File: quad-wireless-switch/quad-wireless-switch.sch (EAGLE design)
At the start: 69 parts, among them IC1 LM2937IMP-3.3, Q1 DN2625K4-G, Q2 SI2323DS-T1-E3, Q3 IRL520, Q4 IRL520, Q5 IRL520, Q6 IRL520, U1 ATMEGA328P_TQFP

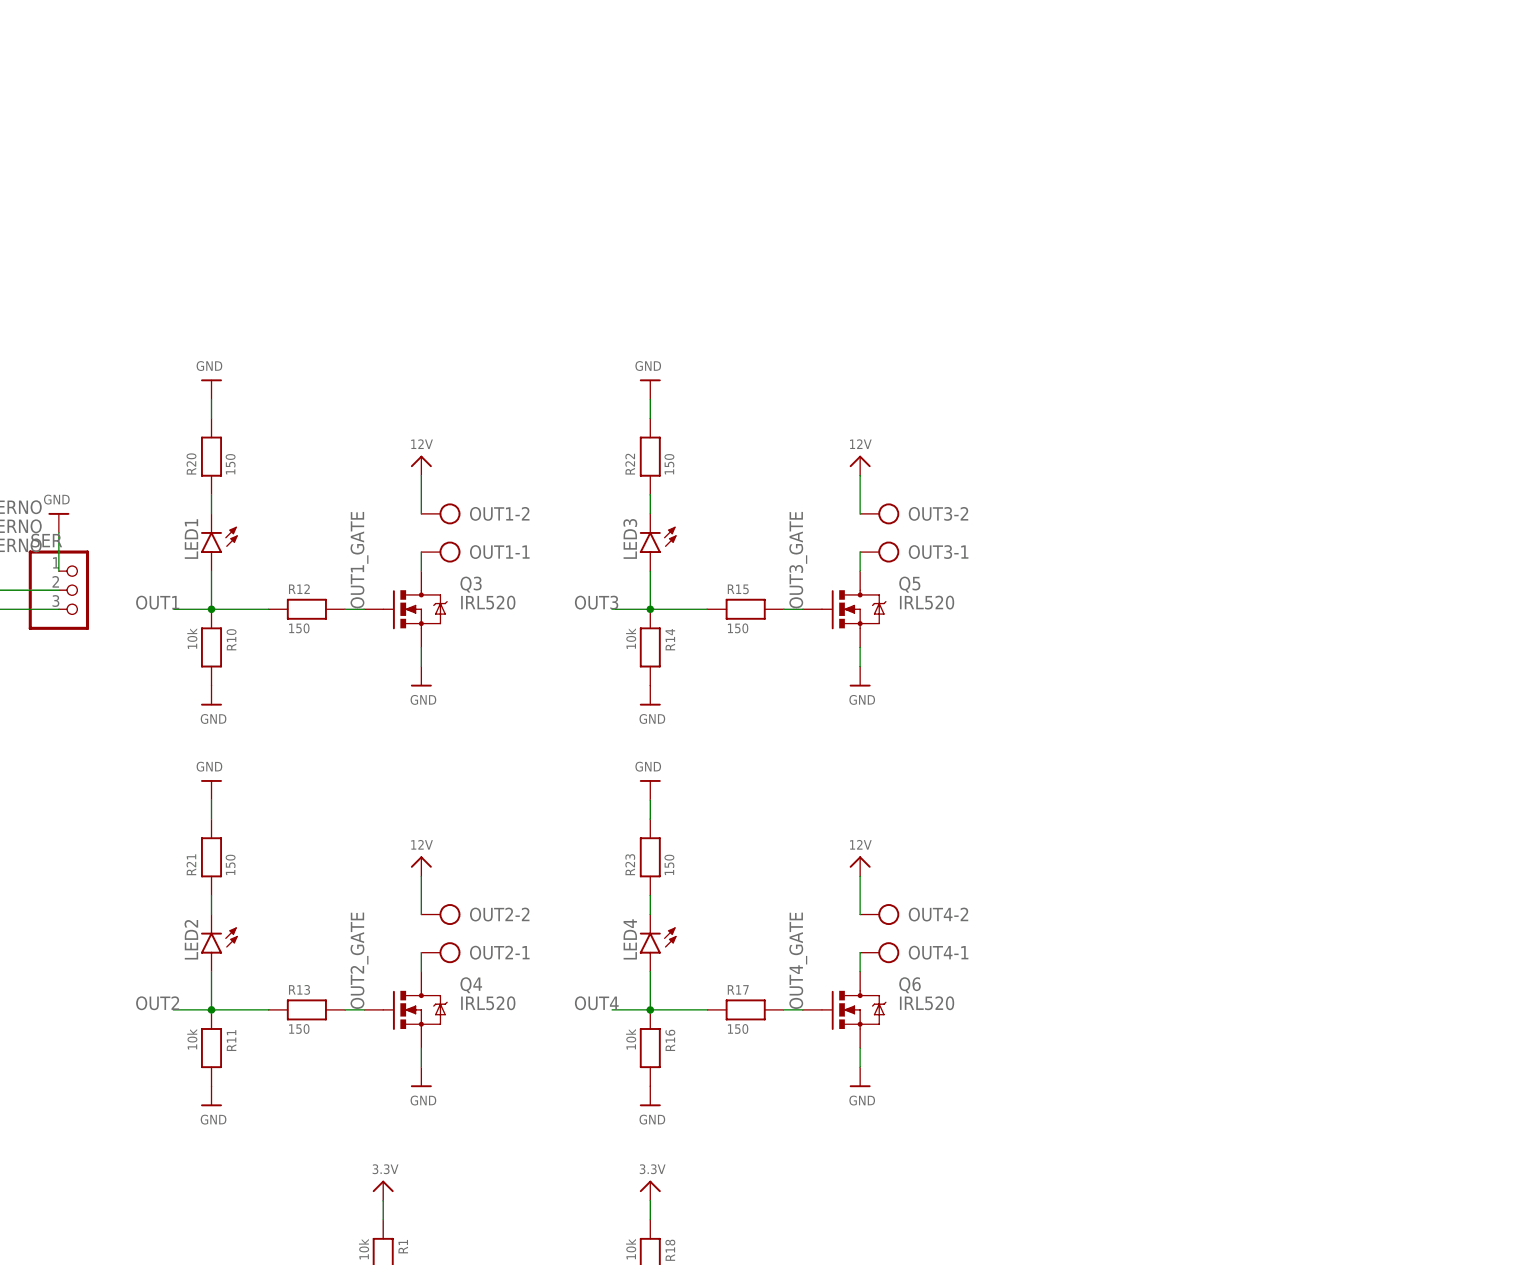
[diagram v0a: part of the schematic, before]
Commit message: quad wireless switch wip
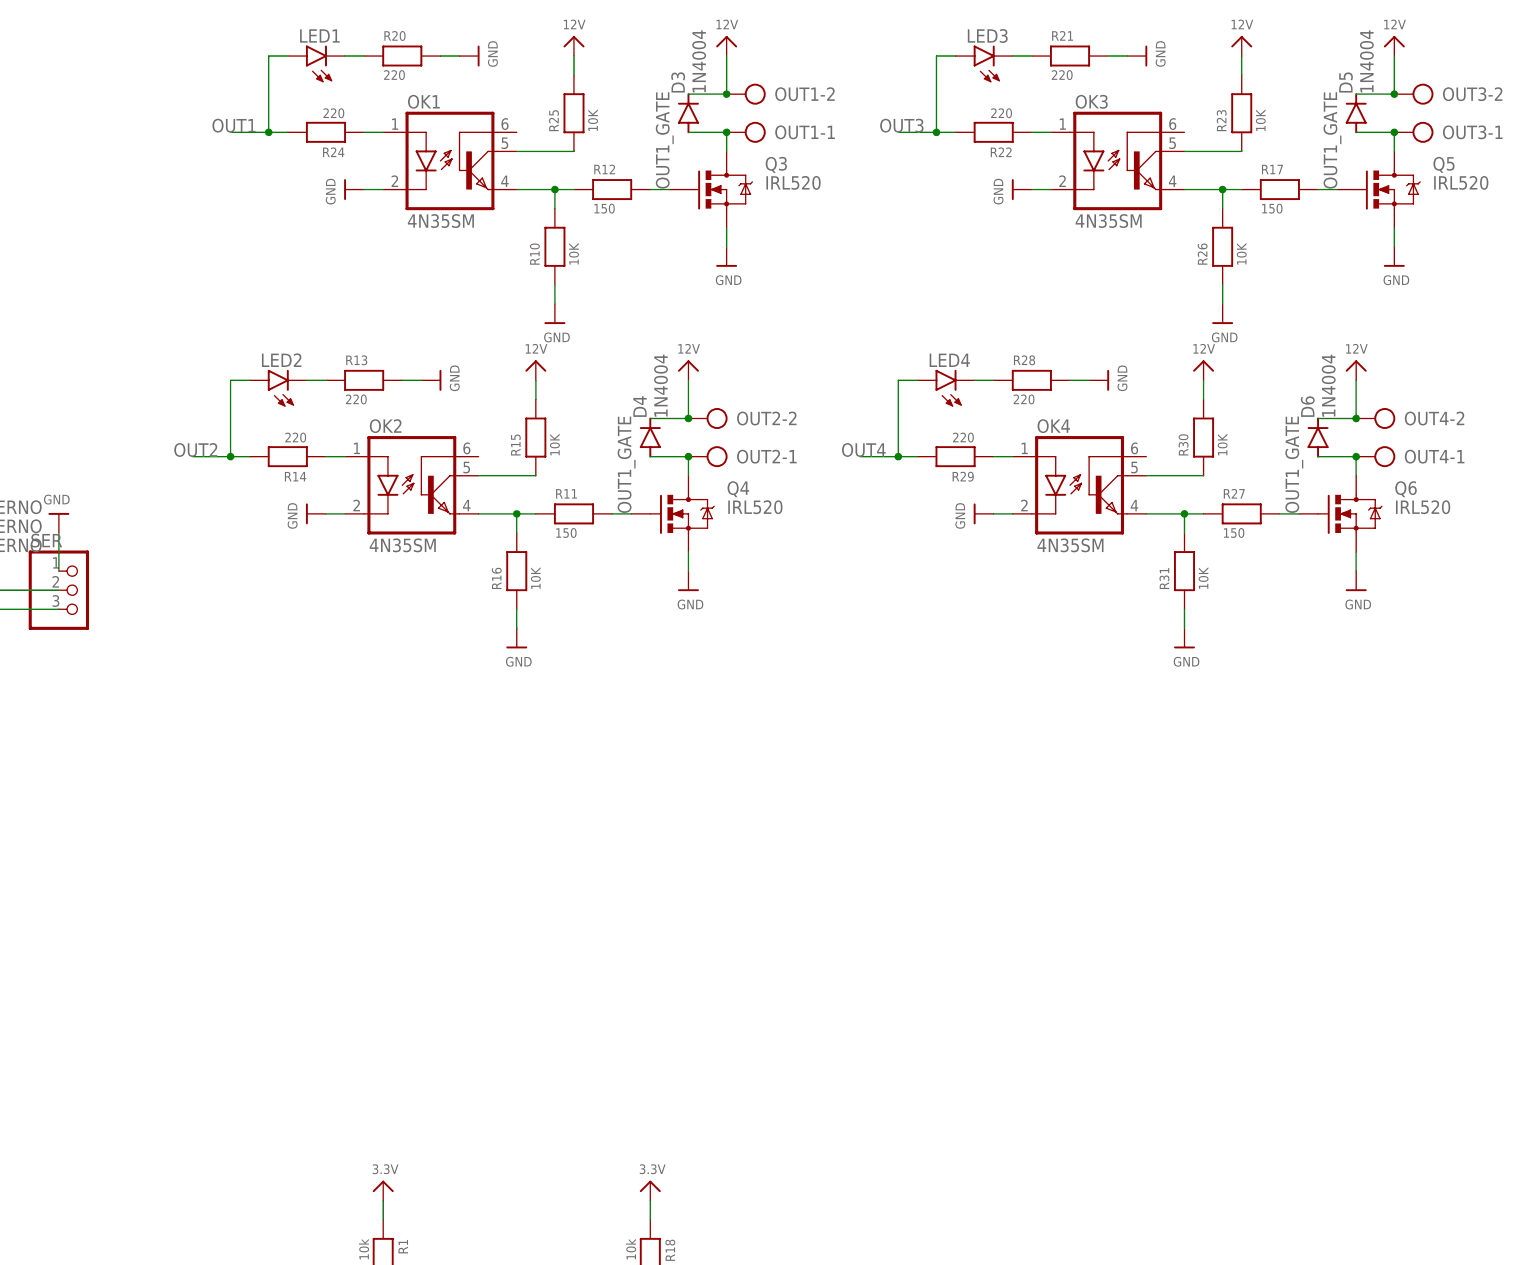
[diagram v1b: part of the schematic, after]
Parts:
- added D3, D4, D5, D6: 1N4004, diode:1N4004
- added OK1, OK2, OK3, OK4: 4N35SM, optocoupler:4N35SM
- added R24, R28, R29: 220, microbuilder:RESISTOR0805
- added R25, R26, R30, R31: 10K, microbuilder:RESISTOR0805
- added R27: 150, microbuilder:RESISTOR0805
- R10, R16: value 10k -> 10K
- R11: value 10k -> 150
- R13, R20, R21, R22: value 150 -> 220
- R14: value 10k -> 220
- R15, R23: value 150 -> 10K
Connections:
- removed net OUT2_GATE: Q4.G, R13.2
- removed net OUT3_GATE: Q5.G, R15.2
- removed net OUT4_GATE: Q6.G, R17.2
- new net N$21: OK1.COL, R25.1
- new net N$23: OK1.A, R24.1
- new net N$24: D5.A, OUT3-1.KL, Q5.D
- new net N$25: LED3.C, R21.1
- new net N$26: OK3.COL, R23.1
- new net N$27: OK3.A, R22.1
- new net N$28: OK3.EMI, R17.1, R26.2
- new net N$29: D6.A, OUT4-1.KL, Q6.D
- new net N$30: LED4.C, R28.1
- new net N$31: OK4.COL, R30.1
- new net N$32: OK4.A, R29.1
- new net N$33: OK4.EMI, R27.1, R31.2
- net 12V: now also D3.C, D4.C, D5.C, D6.C, R15.2, R23.2, R25.2, R30.2
- net GND: now also OK1.C, OK2.C, OK3.C, OK4.C, R10.1, R13.2, R16.1, R26.1, R28.2, R31.1; no longer R10.2, R11.2, R14.2, R16.2, R22.2, R23.2
- net N$18: now also OK2.A, R14.1; no longer OUT3-1.KL, Q5.D
- net N$2: now also OK1.EMI, R10.2, R12.1; no longer LED2.C, R21.1
- net N$22: now also OK2.EMI, R11.1, R16.2; no longer OUT4-1.KL, Q6.D
- net N$3: now also D4.A, OUT2-1.KL, Q4.D; no longer LED3.C, R22.1
- net N$4: now also LED2.C, R13.1; no longer LED4.C, R23.1
- net N$6: now also D3.A
- net N$8: now also OK2.COL, R15.1; no longer OUT2-1.KL, Q4.D
- net OUT1: now also R24.2; no longer R10.1, R12.1
- net OUT1_GATE: now also Q4.G, Q5.G, Q6.G, R11.2, R17.2, R27.2
- net OUT2: now also R14.2; no longer R11.1, R13.1
- net OUT3: now also R22.2; no longer R14.1, R15.1
- net OUT4: now also R29.2; no longer R16.1, R17.1
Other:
- moved on the sheet: LED1, LED2, LED3, LED4, OUT1-1, OUT1-2, OUT2-1, OUT2-2, OUT3-1, OUT3-2, OUT4-1, OUT4-2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
